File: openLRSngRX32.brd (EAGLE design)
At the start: 43 x 39.4 mm, 58 parts, among them IC1 STM32F10XCXT6, IC2 REG1117, U1 MPU-6000QFN-24, Y1 8MHz

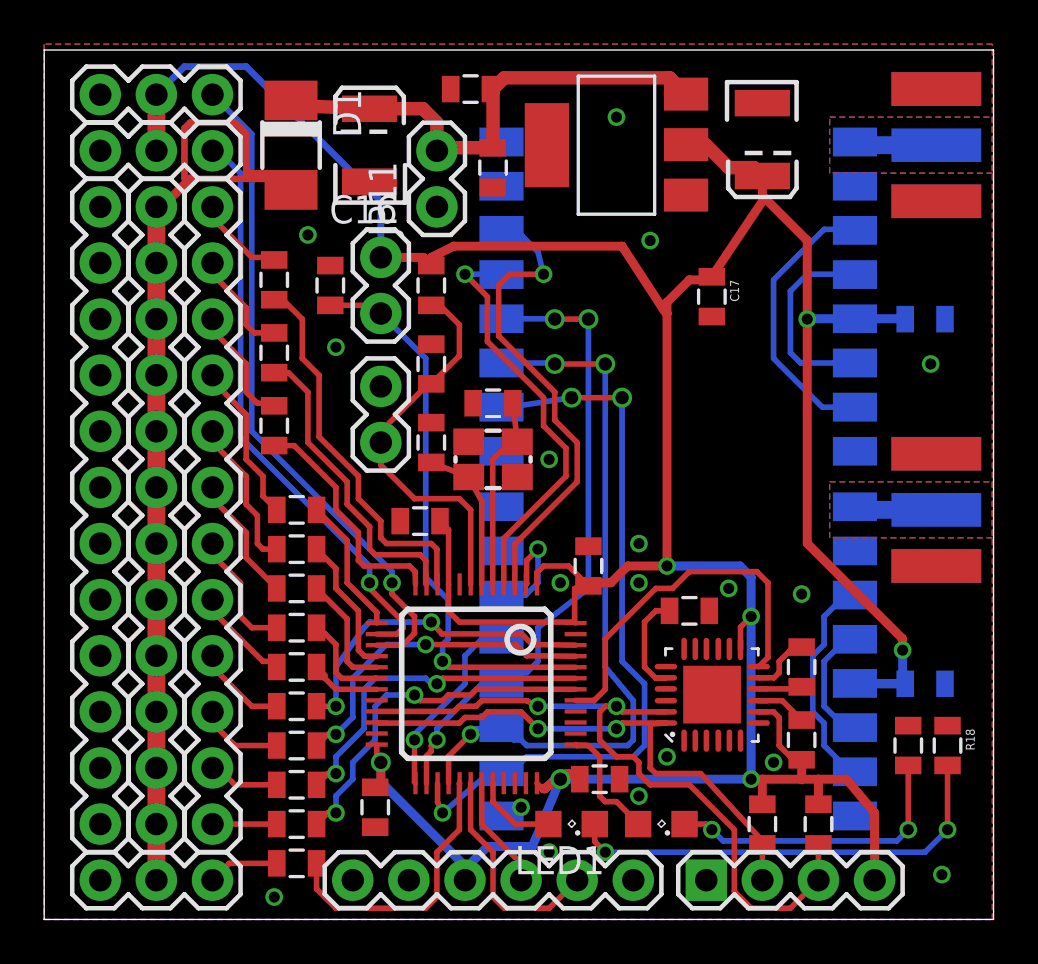
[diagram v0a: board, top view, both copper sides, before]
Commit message: cleanup
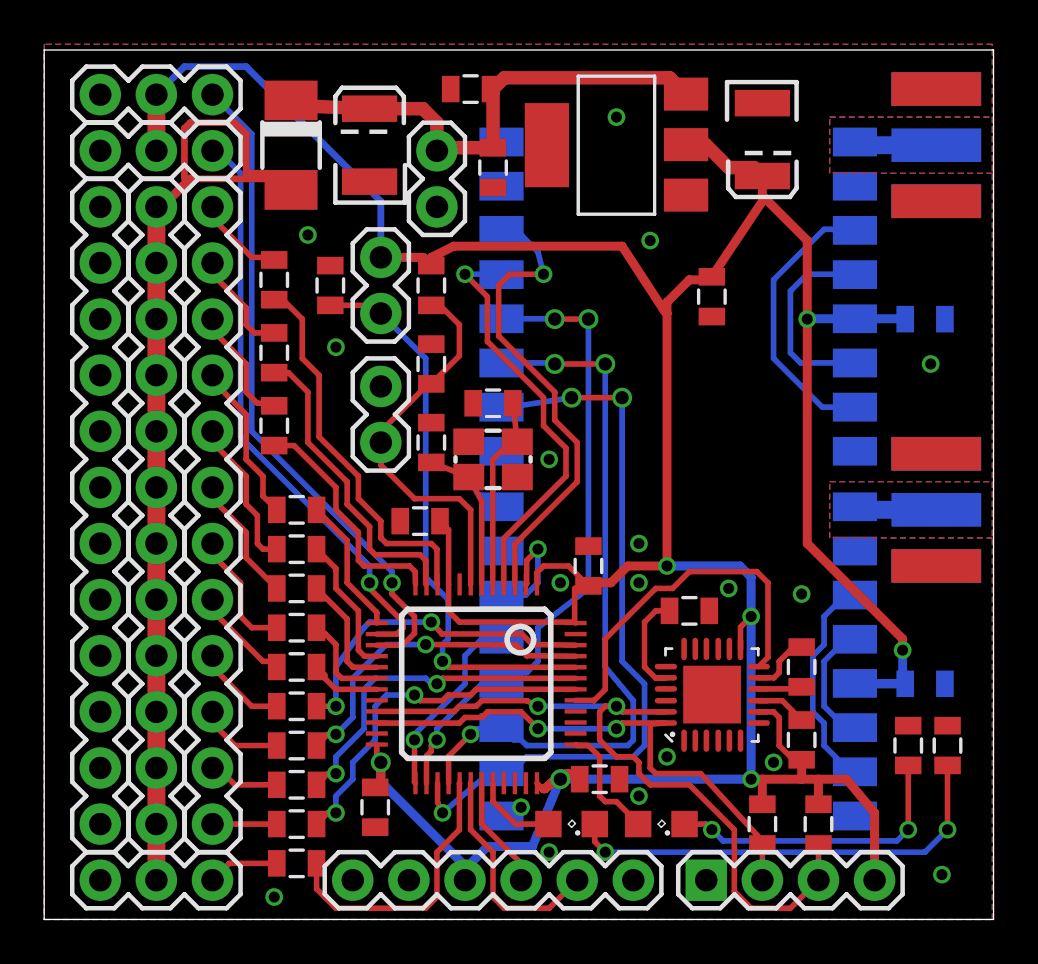
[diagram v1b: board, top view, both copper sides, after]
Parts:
- LED1: value (none) -> RED
- LED2: value (none) -> GREEN
